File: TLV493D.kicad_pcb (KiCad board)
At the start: 2 copper layers, 7 parts, among them J1 Conn_01x04_Female, U1 TLV493D

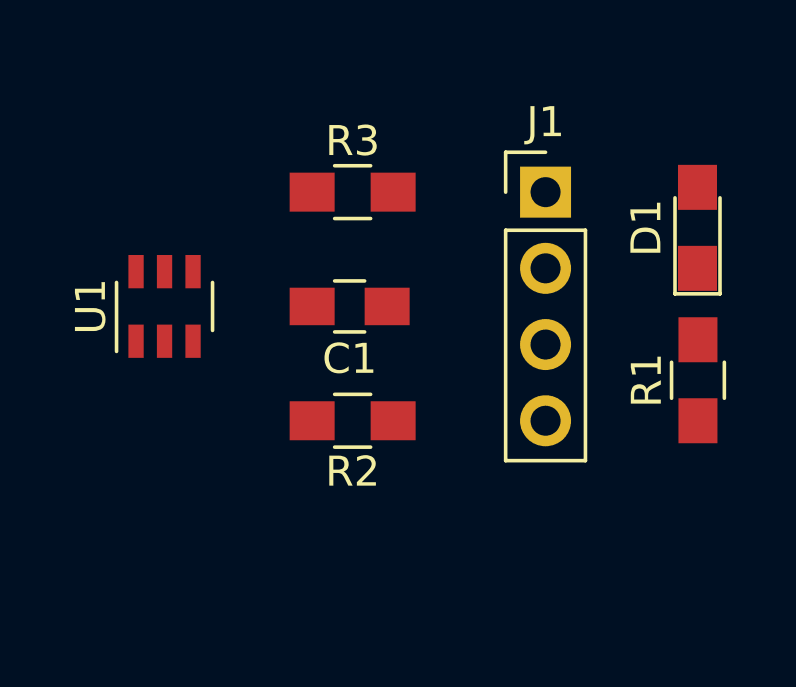
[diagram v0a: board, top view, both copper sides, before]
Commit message: rotate pcb
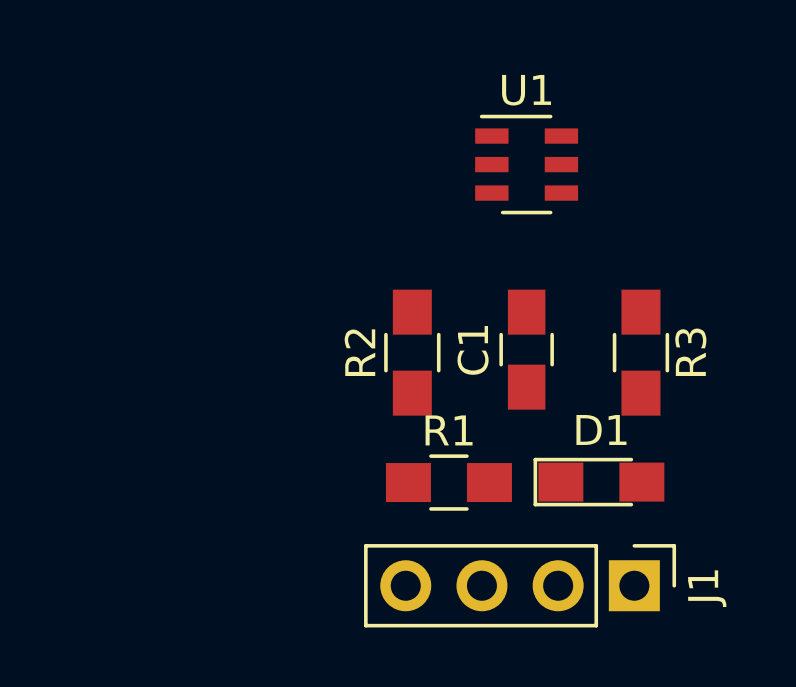
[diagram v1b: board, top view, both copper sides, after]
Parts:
- moved J1 13.4 mm to (157.9, 116.0), turned to 270 degrees
- moved U1 13.0 mm to (154.3, 102.0), turned to 0 degrees
- moved R3 11.0 mm to (158.1, 108.2), turned to 270 degrees
- moved D1 9.06 mm to (156.8, 112.5), turned to 0 degrees
- moved R1 8.97 mm to (151.7, 112.5), turned to 0 degrees
- moved C1 6.07 mm to (154.3, 108.1), turned to 90 degrees
- moved R2 3.02 mm to (150.5, 108.2), turned to 90 degrees
